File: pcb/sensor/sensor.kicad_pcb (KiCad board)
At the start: 2 copper layers, 163.2 x 35 mm, 35 parts, among them J1 Conn_01x05, J2 Conn_01x05, SW1 B, SW10 D, SW11 C#, SW12 C, SW2 A#, SW3 A, SW4 G#, SW5 G, SW6 F#, SW7 F, SW8 E, SW9 D#, U1 74HC165, U2 74HC165

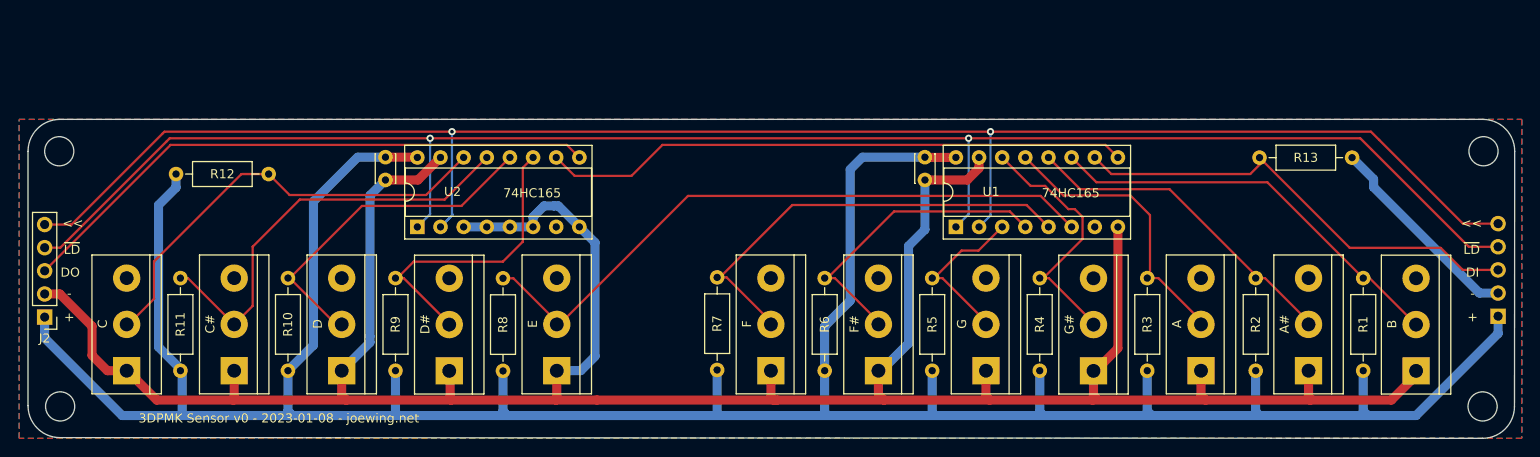
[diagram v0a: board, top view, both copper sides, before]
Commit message: Sensor v0
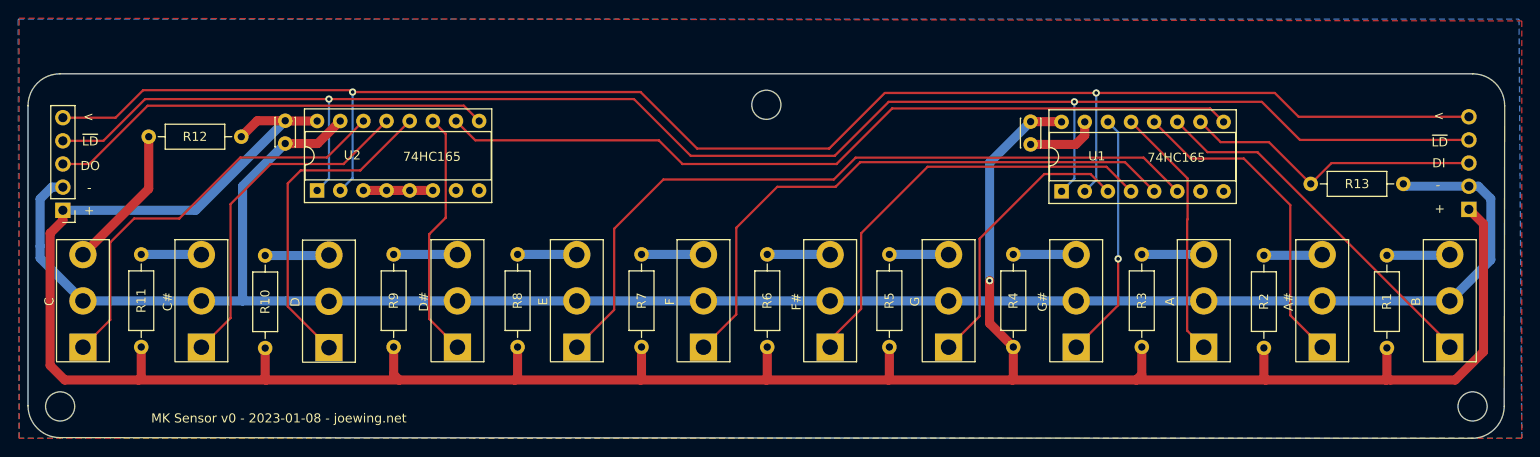
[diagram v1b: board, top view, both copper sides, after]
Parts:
- removed H4: MountingHole, MountingHole:MountingHole_3.2mm_M3
- R13: value 10k -> 100k
- SW1, SW10, SW11, SW12, SW2, SW3, SW4, SW5, SW6, SW7, SW8, SW9: footprint TerminalBlock:TerminalBlock_bornier-3_P5.08mm -> Button_Switch_THT:Mini Limit Switch
- moved H3 77.8 mm to (145.4, 86.1)
- moved U1 12.2 mm to (177.8, 95.6)
- moved C2 12.2 mm to (174.4, 88.0)
- moved J1 12.2 mm to (222.5, 97.6)
- moved J2 11.9 mm to (68.2, 97.7)
- moved C1 11.7 mm to (92.6, 87.8)
- moved U2 11.7 mm to (96.1, 95.5)
- moved R7 8.67 mm to (131.7, 112.7)
- moved R12 8.25 mm to (87.8, 89.6), turned to 180 degrees
- moved SW7 7.84 mm to (138.5, 112.7)
- moved R6 6.82 mm to (145.5, 112.7)
- moved R13 6.31 mm to (215.3, 94.8)
- moved SW6 5.89 mm to (152.4, 112.7)
- moved SW12 5.45 mm to (70.4, 112.7)
- moved R5 5.37 mm to (158.9, 112.7)
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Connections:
- R1 pad 2: Net-(R1-Pad2) -> Net-(SW1-Pad1)
- R11 pad 2: Net-(R11-Pad2) -> Net-(SW11-Pad1)
- R12 pad 2: Net-(R12-Pad2) -> Net-(SW12-Pad1)
- R5 pad 2: Net-(R5-Pad2) -> Net-(SW5-Pad1)
- R6 pad 2: Net-(R6-Pad2) -> Net-(SW6-Pad1)
- R8 pad 2: Net-(R8-Pad2) -> Net-(SW8-Pad1)
- SW1 pad 1: GND -> Net-(SW1-Pad1)
- SW1 pad 2: Net-(R1-Pad2) -> Net-(U1-Pad11)
- SW1 pad 3: (no net) -> GND
- SW10 pad 1: GND -> Net-(R10-Pad2)
- SW10 pad 2: Net-(R10-Pad2) -> Net-(U2-Pad12)
- SW10 pad 3: (no net) -> GND
- SW11 pad 1: GND -> Net-(SW11-Pad1)
- SW11 pad 2: Net-(R11-Pad2) -> Net-(U2-Pad13)
- SW11 pad 3: (no net) -> GND
- SW12 pad 1: GND -> Net-(SW12-Pad1)
- SW12 pad 2: Net-(R12-Pad2) -> Net-(U2-Pad14)
- SW12 pad 3: (no net) -> GND
- SW2 pad 1: GND -> Net-(R2-Pad2)
- SW2 pad 2: Net-(R2-Pad2) -> Net-(U1-Pad12)
- SW2 pad 3: (no net) -> GND
- SW3 pad 1: GND -> Net-(R3-Pad2)
- SW3 pad 2: Net-(R3-Pad2) -> Net-(U1-Pad13)
- SW3 pad 3: (no net) -> GND
- SW4 pad 1: GND -> Net-(R4-Pad2)
- SW4 pad 2: Net-(R4-Pad2) -> Net-(U1-Pad14)
- SW4 pad 3: (no net) -> GND
- SW5 pad 1: GND -> Net-(SW5-Pad1)
- SW5 pad 2: Net-(R5-Pad2) -> Net-(U1-Pad3)
- SW5 pad 3: (no net) -> GND
- SW6 pad 1: GND -> Net-(SW6-Pad1)
- SW6 pad 2: Net-(R6-Pad2) -> Net-(U1-Pad4)
- SW6 pad 3: (no net) -> GND
- SW7 pad 1: GND -> Net-(R7-Pad2)
- SW7 pad 2: Net-(R7-Pad2) -> Net-(U1-Pad5)
- SW7 pad 3: (no net) -> GND
- SW8 pad 1: GND -> Net-(SW8-Pad1)
- SW8 pad 2: Net-(R8-Pad2) -> Net-(U1-Pad6)
- SW8 pad 3: (no net) -> GND
- SW9 pad 1: GND -> Net-(R9-Pad2)
- SW9 pad 2: Net-(R9-Pad2) -> Net-(U2-Pad11)
- SW9 pad 3: (no net) -> GND
- U1 pad 11: Net-(R1-Pad2) -> Net-(U1-Pad11)
- U1 pad 12: Net-(R2-Pad2) -> Net-(U1-Pad12)
- U1 pad 13: Net-(R3-Pad2) -> Net-(U1-Pad13)
- U1 pad 14: Net-(R4-Pad2) -> Net-(U1-Pad14)
- U1 pad 3: Net-(R5-Pad2) -> Net-(U1-Pad3)
- U1 pad 4: Net-(R6-Pad2) -> Net-(U1-Pad4)
- U1 pad 5: Net-(R7-Pad2) -> Net-(U1-Pad5)
- U1 pad 6: Net-(R8-Pad2) -> Net-(U1-Pad6)
- U2 pad 11: Net-(R9-Pad2) -> Net-(U2-Pad11)
- U2 pad 12: Net-(R10-Pad2) -> Net-(U2-Pad12)
- U2 pad 13: Net-(R11-Pad2) -> Net-(U2-Pad13)
- U2 pad 14: Net-(R12-Pad2) -> Net-(U2-Pad14)
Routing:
- net GND: track 327.5 -> 231.2 mm
- net Net-(U1-Pad6): track 0.00 -> 81.3 mm
- net Net-(R8-Pad2): track 71.5 -> 0.00 mm
- net Net-(U1-Pad5): track 0.00 -> 64.8 mm
- net Net-(R12-Pad2): track 48.7 -> 0.00 mm
- net Net-(U1-Pad4): track 0.00 -> 47.7 mm
- net Net-(R11-Pad2): track 47.1 -> 0.00 mm
- net Net-(U2-Pad14): track 0.00 -> 46.0 mm
- net Net-(R1-Pad2): track 45.4 -> 0.00 mm
- net Net-(R7-Pad2): track 48.4 -> 6.81 mm
- net Net-(U1-Pad11): track 0.00 -> 40.3 mm
- net Net-(U2-Pad13): track 0.00 -> 37.9 mm
- net Net-(U2-Pad12): track 0.00 -> 36.1 mm
- net Net-(U1-Pad12): track 0.00 -> 35.8 mm
- net Net-(R6-Pad2): track 33.5 -> 0.00 mm
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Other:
- board size 163.2 x 35 mm -> 162.1 x 40 mm
- board text added: "<"
- board text added: "MK Sensor v0 - 2023-01-08 - joewing.net"
- board text removed: "3DPMK Sensor v0 - 2023-01-08 - joewing.net"
- board text removed: "<<"
